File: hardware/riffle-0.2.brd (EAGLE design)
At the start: 98.5 x 18 mm, 35 parts, among them IC1 ATMEGA328P, IC2 MCP73831, IC3 CH340G, IC4 MCP1700-33, IC5 24AA128SN, J1 AYZ0202, X1 USBSMD, X2 12MHz, X3 16 MHz

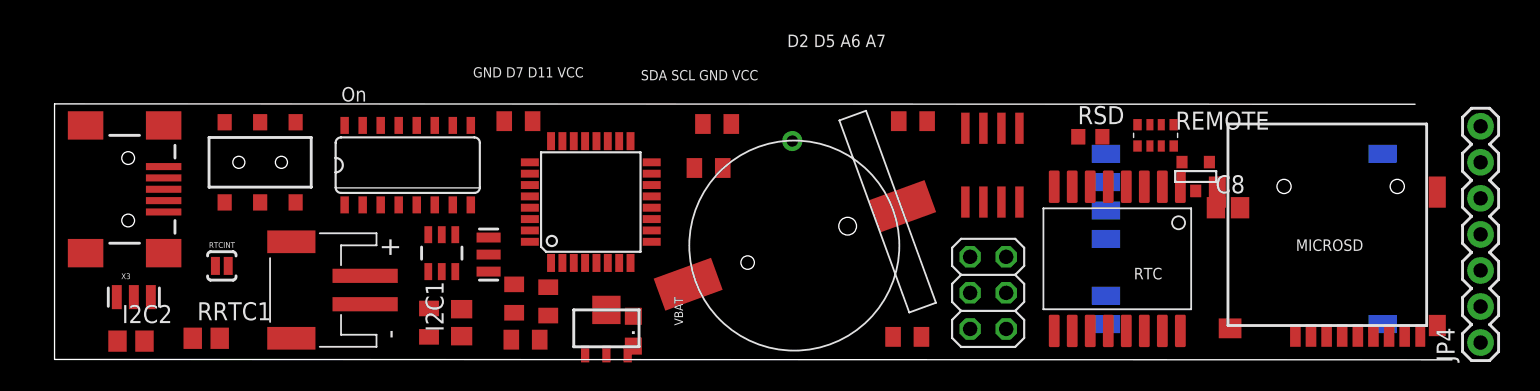
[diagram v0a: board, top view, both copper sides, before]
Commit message: update
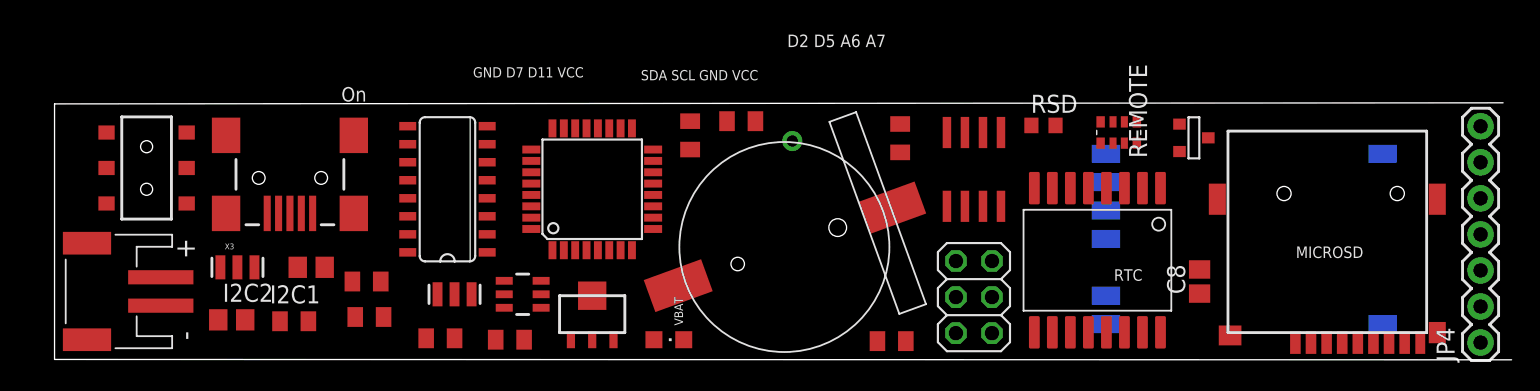
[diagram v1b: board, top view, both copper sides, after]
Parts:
- removed RRTC1: 10K, rcl:R0805
- removed RTCINT: SOLDERJUMPERNO, _SparkFun:SJ_2S-NO
- moved C5 17.3 mm to (22.7, 10.3)
- moved CN1 14.4 mm to (4.30, 12.1)
- moved X1 11.4 mm to (17.1, 20.1), turned to 270 degrees
- moved I2C1 11.3 mm to (18.6, 13.8), turned to 180 degrees
- moved RRST 10.5 mm to (22.5, 12.8), turned to 0 degrees
- moved C4 9.50 mm to (17.4, 10.0), turned to 180 degrees
- moved J1 8.01 mm to (7.00, 20.8), turned to 90 degrees
- moved X3 7.60 mm to (13.4, 13.8)
- moved I2C2 7.26 mm to (13.0, 10.1)
- moved IC2 6.40 mm to (33.5, 11.9), turned to 270 degrees
- moved C1 6.00 mm to (27.7, 8.80)
- moved C8 5.57 mm to (81.2, 12.8), turned to 90 degrees
- moved RC 4.02 mm to (48.9, 24.1)
- moved C7 3.82 mm to (32.6, 8.70), turned to 180 degrees
- moved X2 3.69 mm to (28.7, 11.9), turned to 0 degrees
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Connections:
- removed net N$4: RRTC1.2, RTC.3, RTCINT.1
- net D3: no longer RTCINT.2
- net VCC: no longer RRTC1.1
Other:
- board size 98.5 x 18 mm -> 102.7 x 18.1 mm

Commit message: update
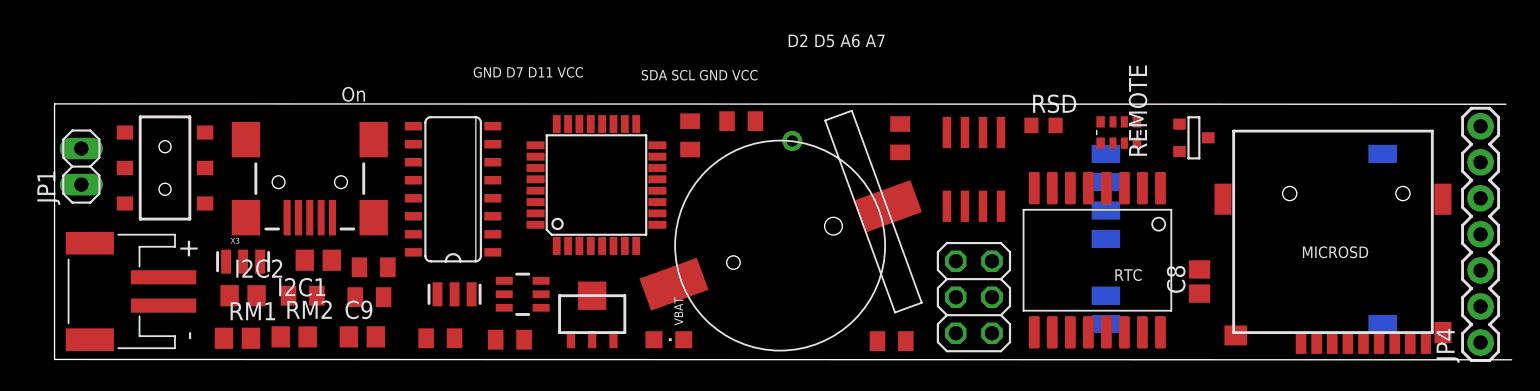
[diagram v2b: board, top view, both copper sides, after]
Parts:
- added C9: .1uF, rcl:C0805@1
- added JP1: (no value), pinhead:1X02
- added RM1, RM2: 10K, rcl:R0805
- moved C4 1.90 mm to (18.0, 11.8)
- moved I2C2 1.88 mm to (13.8, 11.8)
- moved X1 1.43 mm to (18.5, 19.8)
- moved C5 1.40 mm to (22.7, 11.7)
- moved J1 1.30 mm to (8.30, 20.8)
- moved RRST 1.12 mm to (23.0, 13.8)
- moved I2C1 0.71 mm to (19.1, 14.3)
- moved X3 0.57 mm to (13.8, 14.2)
- moved IC1 0.42 mm to (38.7, 19.6)
- moved IC3 0.40 mm to (28.6, 19.3)
- moved MICROSD 0.40 mm to (90.6, 19.0)
- moved BAT 0.32 mm to (55.4, 16.7)
- moved CN1 0.20 mm to (4.50, 12.1)
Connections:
- new net VIN: RM1.2
- net A3: now also C9.2, RM1.1, RM2.2
- net GND: now also C9.1, RM2.1
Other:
- board size 102.7 x 18.1 mm -> 102.7 x 18 mm
